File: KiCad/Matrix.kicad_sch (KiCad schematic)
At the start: 0 parts

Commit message: "finish" the keyboard schematics
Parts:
- added D1: ESC, symbol Device:D
- added D10: F9, symbol Device:D
- added D11: F10, symbol Device:D
- added D12: F11, symbol Device:D
- added D13: F12, symbol Device:D
- added D14: Del, symbol Device:D
- added D15: Ins, symbol Device:D
- added D16: `/~, symbol Device:D
- added D17: 1, symbol Device:D
- added D18: 2, symbol Device:D
- added D19: 3, symbol Device:D
- added D2: F1, symbol Device:D
- added D20: 4, symbol Device:D
- added D21: 5, symbol Device:D
- added D22: 6, symbol Device:D
- added D23: 7, symbol Device:D
- added D24: 8, symbol Device:D
- added D25: 9, symbol Device:D
- added D26: 0, symbol Device:D
- added D27: -, symbol Device:D
- added D28: +, symbol Device:D
- added D29: Backspace, symbol Device:D
- added D3: F2, symbol Device:D
- added D30: End, symbol Device:D
- added D31: Tab, symbol Device:D
- added D32: Q, symbol Device:D
- added D33: W, symbol Device:D
- added D34: E, symbol Device:D
- added D35: R, symbol Device:D
- added D36: T, symbol Device:D
- added D37: Y, symbol Device:D
- added D38: U, symbol Device:D
- added D39: I, symbol Device:D
- added D4: F3, symbol Device:D
- added D40: O, symbol Device:D
- added D41: P, symbol Device:D
- added D42: [, symbol Device:D
- added D43: ], symbol Device:D
- added D44: \, symbol Device:D
- added D45: PgUp, symbol Device:D
- added D46: CapsLock, symbol Device:D
- added D47: A, symbol Device:D
- added D48: S, symbol Device:D
- added D49: D, symbol Device:D
- added D5: F4, symbol Device:D
- added D50: F, symbol Device:D
- added D51: G, symbol Device:D
- added D52: H, symbol Device:D
- added D53: J, symbol Device:D
- added D54: K, symbol Device:D
- added D55: L, symbol Device:D
- added D56: ;, symbol Device:D
- added D57: ', symbol Device:D
- added D58: Enter, symbol Device:D
- added D59: PgDn, symbol Device:D
- added D6: F5, symbol Device:D
- added D60: LShift, symbol Device:D
- added D61: Z, symbol Device:D
- added D62: X, symbol Device:D
- added D63: C, symbol Device:D
- added D64: V, symbol Device:D
- added D65: B, symbol Device:D
- added D66: N, symbol Device:D
- added D67: M, symbol Device:D
- added D68: ,, symbol Device:D
- added D69: ., symbol Device:D
- added D7: F6, symbol Device:D
- added D70: /, symbol Device:D
- added D71: RShift, symbol Device:D
- added D72: Up, symbol Device:D
- added D73: Home, symbol Device:D
- added D74: LCtrl, symbol Device:D
- added D75: Win, symbol Device:D
- added D76, D78: Alt, symbol Device:D
- added D77: Space, symbol Device:D
- added D79: FN, symbol Device:D
- added D8: F7, symbol Device:D
- added D80: RCtrl, symbol Device:D
- added D81: Right, symbol Device:D
- added D82: Down, symbol Device:D
- added D83: Left, symbol Device:D
- added D9: F8, symbol Device:D
- added MX1, MX10, MX11, MX12, MX13, MX14, MX15, MX16, MX17, MX18, MX19, MX2, MX20, MX21, MX22, MX23, MX24, MX25, MX26, MX27, MX28, MX29, MX3, MX30, MX31, MX32, MX33, MX34, MX35, MX36, MX37, MX38, MX39, MX4, MX40, MX41, MX42, MX43, MX44, MX45, MX46, MX47, MX48, MX49, MX5, MX50, MX51, MX52, MX53, MX54, MX55, MX56, MX57, MX58, MX59, MX6, MX60, MX61, MX62, MX63, MX64, MX65, MX66, MX67, MX68, MX69, MX7, MX70, MX71, MX72, MX73, MX74, MX75, MX76, MX8, MX80, MX83, MX84, MX85, MX86, MX87, MX88, MX9: MX-NoLED, symbol MX_Alps_Hybrid:MX-NoLED
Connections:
- new net: D60.2 (A), MX59.2 (ROW)
- new net: D50.2 (A), MX50.2 (ROW)
- new net: D77.2 (A), MX80.2 (ROW)
- new net: D15.2 (A), MX15.2 (ROW)
- new net: D11.2 (A), MX11.2 (ROW)
- new net: D31.2 (A), MX31.2 (ROW)
- new net: D32.2 (A), MX32.2 (ROW)
- new net: D82.2 (A), MX87.2 (ROW)
- new net: D38.2 (A), MX38.2 (ROW)
- new net: D67.2 (A), MX67.2 (ROW)
- new net: D53.2 (A), MX53.2 (ROW)
- new net: D46.2 (A), MX46.2 (ROW)
- new net: D40.2 (A), MX40.2 (ROW)
- new net: D63.2 (A), MX63.2 (ROW)
- new net: D8.2 (A), MX8.2 (ROW)
- new net: D41.2 (A), MX41.2 (ROW)
- new net: D7.2 (A), MX7.2 (ROW)
- new net: D83.2 (A), MX88.2 (ROW)
- new net: D13.2 (A), MX13.2 (ROW)
- new net: D37.2 (A), MX37.2 (ROW)
- new net: D59.2 (A), MX60.2 (ROW)
- new net: D52.2 (A), MX52.2 (ROW)
- new net: D24.2 (A), MX24.2 (ROW)
- new net: D2.2 (A), MX2.2 (ROW)
- new net: D14.2 (A), MX14.2 (ROW)
- new net: D76.2 (A), MX76.2 (ROW)
- new net: D45.2 (A), MX45.2 (ROW)
- new net: D73.2 (A), MX74.2 (ROW)
- new net: D81.2 (A), MX86.2 (ROW)
- new net: D17.2 (A), MX17.2 (ROW)
- new net: D75.2 (A), MX75.2 (ROW)
- new net: D65.2 (A), MX65.2 (ROW)
- new net: D74.2 (A), MX71.2 (ROW)
- new net: D48.2 (A), MX48.2 (ROW)
- new net: D71.2 (A), MX72.2 (ROW)
- new net: D10.2 (A), MX10.2 (ROW)
- new net: D33.2 (A), MX33.2 (ROW)
- new net: D30.2 (A), MX30.2 (ROW)
- new net: D51.2 (A), MX51.2 (ROW)
- new net: D4.2 (A), MX4.2 (ROW)
- new net: D21.2 (A), MX21.2 (ROW)
- new net: D58.2 (A), MX58.2 (ROW)
- new net: D64.2 (A), MX64.2 (ROW)
- new net: D1.2 (A), MX1.2 (ROW)
- new net: D44.2 (A), MX44.2 (ROW)
- new net: D36.2 (A), MX36.2 (ROW)
- new net: D47.2 (A), MX47.2 (ROW)
- new net: D54.2 (A), MX54.2 (ROW)
- new net: D72.2 (A), MX73.2 (ROW)
- new net: D62.2 (A), MX62.2 (ROW)
- new net: D18.2 (A), MX18.2 (ROW)
- new net: D66.2 (A), MX66.2 (ROW)
- new net: D6.2 (A), MX6.2 (ROW)
- new net: D25.2 (A), MX25.2 (ROW)
- new net: D68.2 (A), MX68.2 (ROW)
- new net: D34.2 (A), MX34.2 (ROW)
- new net: D35.2 (A), MX35.2 (ROW)
- new net: D55.2 (A), MX55.2 (ROW)
- new net: D16.2 (A), MX16.2 (ROW)
- new net: D27.2 (A), MX27.2 (ROW)
- new net: D57.2 (A), MX57.2 (ROW)
- new net: D28.2 (A), MX28.2 (ROW)
- new net: D9.2 (A), MX9.2 (ROW)
- new net: D39.2 (A), MX39.2 (ROW)
- new net: D78.2 (A), MX83.2 (ROW)
- new net: D23.2 (A), MX23.2 (ROW)
- new net: D70.2 (A), MX70.2 (ROW)
- new net: D20.2 (A), MX20.2 (ROW)
- new net: D3.2 (A), MX3.2 (ROW)
- new net: D19.2 (A), MX19.2 (ROW)
- new net: D69.2 (A), MX69.2 (ROW)
- new net: D49.2 (A), MX49.2 (ROW)
- new net: D29.2 (A), MX29.2 (ROW)
- new net: D5.2 (A), MX5.2 (ROW)
- new net: D42.2 (A), MX42.2 (ROW)
- new net: D26.2 (A), MX26.2 (ROW)
- new net: D80.2 (A), MX85.2 (ROW)
- new net: D22.2 (A), MX22.2 (ROW)
- new net: D79.2 (A), MX84.2 (ROW)
- new net: D61.2 (A), MX61.2 (ROW)
- new net: D43.2 (A), MX43.2 (ROW)
- new net: D12.2 (A), MX12.2 (ROW)
- new net: D56.2 (A), MX56.2 (ROW)
- new net col0: MX1.1 (COL), MX16.1 (COL), MX31.1 (COL), MX46.1 (COL), MX59.1 (COL), MX71.1 (COL)
- new net col1: MX17.1 (COL), MX2.1 (COL), MX32.1 (COL), MX47.1 (COL), MX61.1 (COL), MX75.1 (COL)
- new net col10: MX11.1 (COL), MX26.1 (COL), MX41.1 (COL), MX56.1 (COL), MX70.1 (COL), MX84.1 (COL)
- new net col11: MX12.1 (COL), MX27.1 (COL), MX42.1 (COL), MX57.1 (COL), MX85.1 (COL)
- new net col12: MX13.1 (COL), MX28.1 (COL), MX43.1 (COL), MX58.1 (COL), MX72.1 (COL), MX86.1 (COL)
- new net col13: MX14.1 (COL), MX29.1 (COL), MX44.1 (COL), MX73.1 (COL), MX87.1 (COL)
- new net col14: MX15.1 (COL), MX30.1 (COL), MX45.1 (COL), MX60.1 (COL), MX74.1 (COL), MX88.1 (COL)
- new net col2: MX18.1 (COL), MX3.1 (COL), MX33.1 (COL), MX48.1 (COL), MX62.1 (COL), MX76.1 (COL)
- new net col3: MX19.1 (COL), MX34.1 (COL), MX4.1 (COL), MX49.1 (COL), MX63.1 (COL)
- new net col4: MX20.1 (COL), MX35.1 (COL), MX5.1 (COL), MX50.1 (COL), MX64.1 (COL)
- new net col5: MX21.1 (COL), MX36.1 (COL), MX51.1 (COL), MX6.1 (COL), MX65.1 (COL)
- new net col6: MX22.1 (COL), MX37.1 (COL), MX52.1 (COL), MX66.1 (COL), MX7.1 (COL), MX80.1 (COL)
- new net col7: MX23.1 (COL), MX38.1 (COL), MX53.1 (COL), MX67.1 (COL), MX8.1 (COL)
- new net col8: MX24.1 (COL), MX39.1 (COL), MX54.1 (COL), MX68.1 (COL), MX9.1 (COL)
- new net col9: MX10.1 (COL), MX25.1 (COL), MX40.1 (COL), MX55.1 (COL), MX69.1 (COL), MX83.1 (COL)
- new net row0: D1.1 (K), D10.1 (K), D11.1 (K), D12.1 (K), D13.1 (K), D14.1 (K), D15.1 (K), D2.1 (K), D3.1 (K), D4.1 (K), D5.1 (K), D6.1 (K), D7.1 (K), D8.1 (K), D9.1 (K)
- new net row1: D16.1 (K), D17.1 (K), D18.1 (K), D19.1 (K), D20.1 (K), D21.1 (K), D22.1 (K), D23.1 (K), D24.1 (K), D25.1 (K), D26.1 (K), D27.1 (K), D28.1 (K), D29.1 (K), D30.1 (K)
- new net row2: D31.1 (K), D32.1 (K), D33.1 (K), D34.1 (K), D35.1 (K), D36.1 (K), D37.1 (K), D38.1 (K), D39.1 (K), D40.1 (K), D41.1 (K), D42.1 (K), D43.1 (K), D44.1 (K), D45.1 (K)
- new net row3: D46.1 (K), D47.1 (K), D48.1 (K), D49.1 (K), D50.1 (K), D51.1 (K), D52.1 (K), D53.1 (K), D54.1 (K), D55.1 (K), D56.1 (K), D57.1 (K), D58.1 (K), D59.1 (K)
- new net row4: D60.1 (K), D61.1 (K), D62.1 (K), D63.1 (K), D64.1 (K), D65.1 (K), D66.1 (K), D67.1 (K), D68.1 (K), D69.1 (K), D70.1 (K), D71.1 (K), D72.1 (K), D73.1 (K)
- new net row5: D74.1 (K), D75.1 (K), D76.1 (K), D77.1 (K), D78.1 (K), D79.1 (K), D80.1 (K), D81.1 (K), D82.1 (K), D83.1 (K)

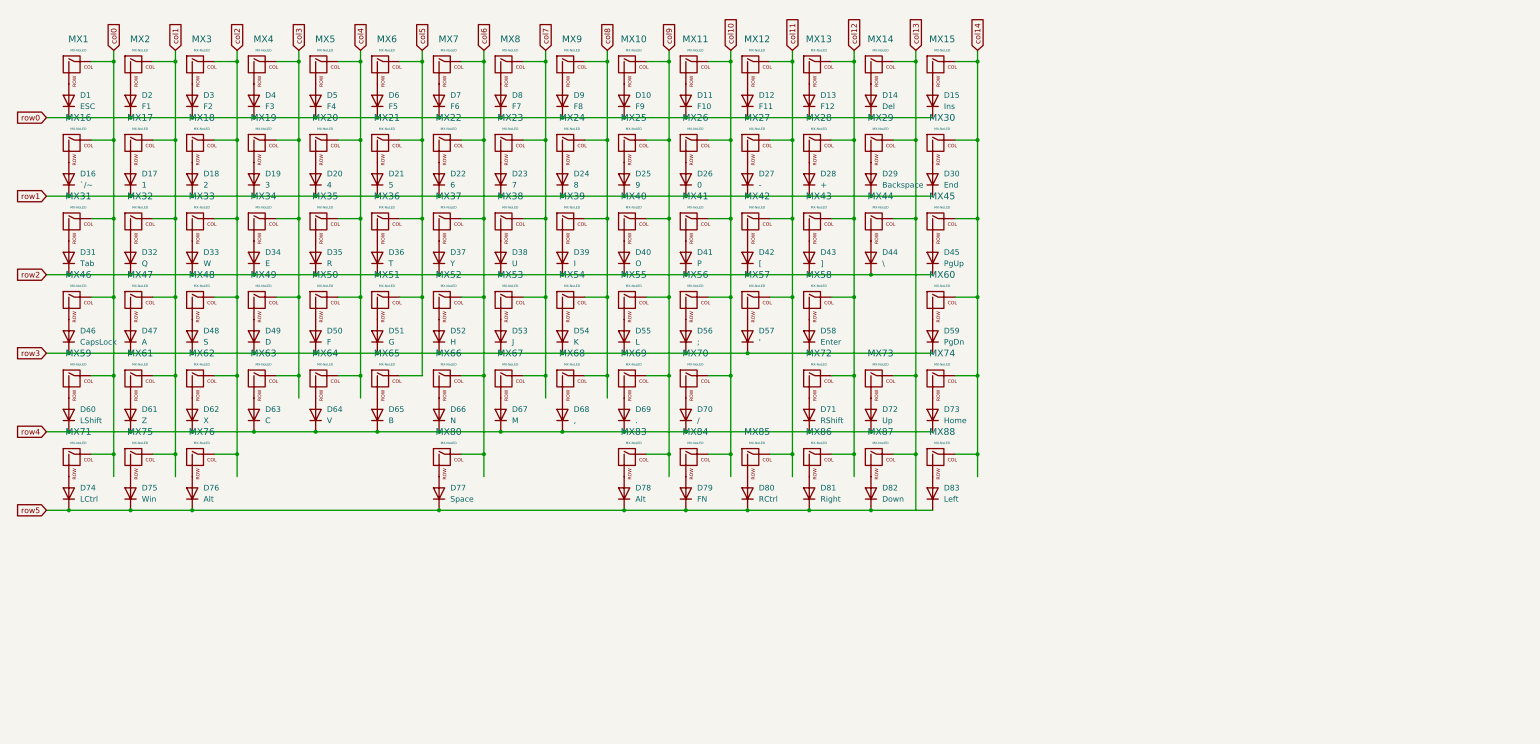
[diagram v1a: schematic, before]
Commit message: fix stuff... i forgot the other stuff i added
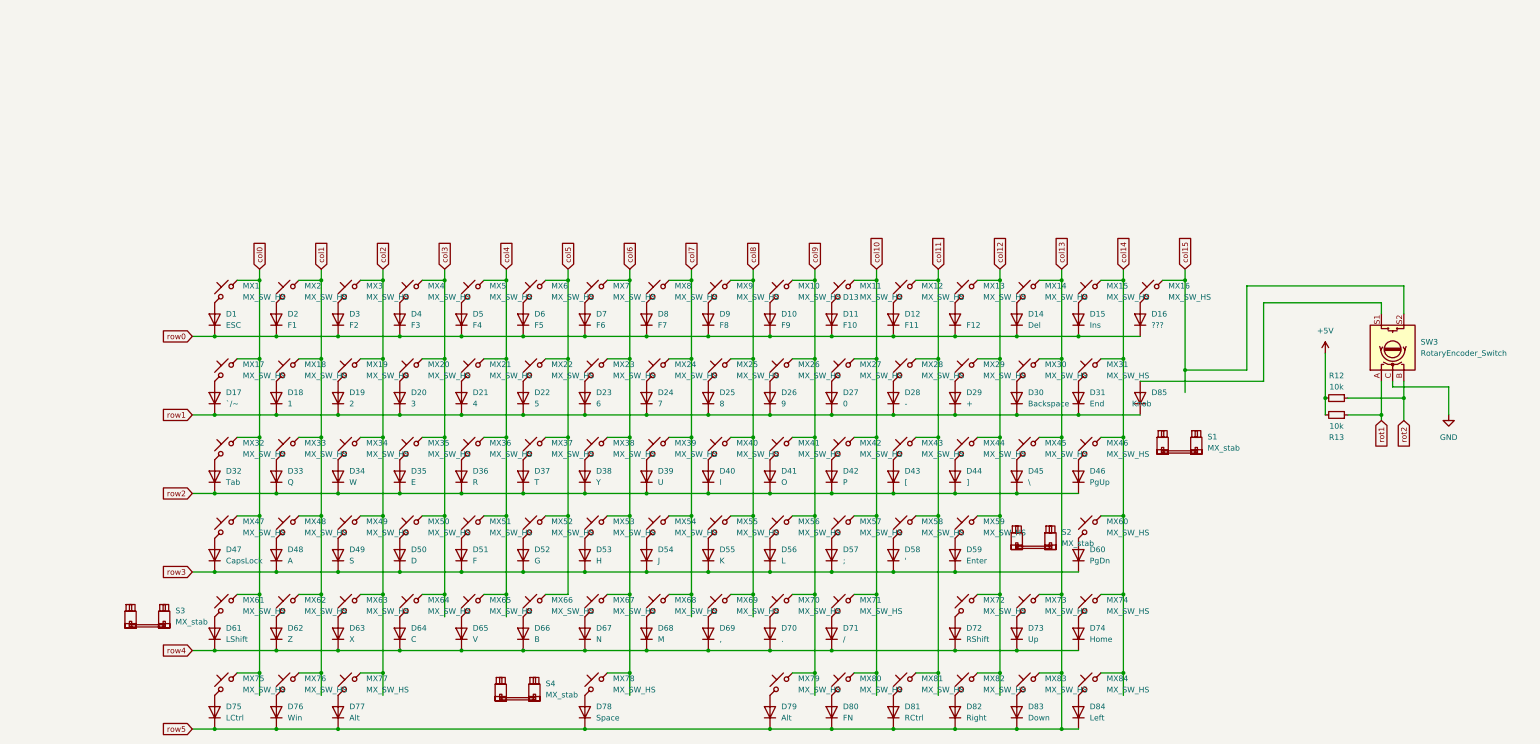
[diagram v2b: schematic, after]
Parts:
- removed MX1, MX10, MX11, MX12, MX13, MX14, MX15, MX16, MX17, MX18, MX19, MX2, MX20, MX21, MX22, MX23, MX24, MX25, MX26, MX27, MX28, MX29, MX3, MX30, MX31, MX32, MX33, MX34, MX35, MX36, MX37, MX38, MX39, MX4, MX40, MX41, MX42, MX43, MX44, MX45, MX46, MX47, MX48, MX49, MX5, MX50, MX51, MX52, MX53, MX54, MX55, MX56, MX57, MX58, MX59, MX6, MX60, MX61, MX62, MX63, MX64, MX65, MX66, MX67, MX68, MX69, MX7, MX70, MX71, MX72, MX73, MX74, MX75, MX76, MX8, MX80, MX83, MX84, MX85, MX86, MX87, MX88, MX9: MX-NoLED, symbol MX_Alps_Hybrid:MX-NoLED
- added D16: ???, Diode_SMD:D_SOD-123, symbol Device:D
- added D85: Knob, Diode_SMD:D_SOD-123, symbol Device:D
- added MX1, MX10, MX11, MX12, MX13, MX14, MX15, MX16, MX17, MX18, MX19, MX2, MX20, MX21, MX22, MX23, MX24, MX25, MX26, MX27, MX28, MX29, MX3, MX30, MX31, MX32, MX33, MX34, MX35, MX36, MX37, MX38, MX39, MX4, MX40, MX41, MX42, MX43, MX44, MX45, MX46, MX47, MX48, MX49, MX5, MX50, MX51, MX52, MX53, MX54, MX55, MX56, MX57, MX58, MX59, MX6, MX60, MX61, MX62, MX63, MX64, MX65, MX66, MX67, MX68, MX69, MX7, MX70, MX71, MX72, MX73, MX74, MX75, MX76, MX77, MX78, MX79, MX8, MX80, MX81, MX82, MX83, MX84, MX9: MX_SW_HS, PCM_marbastlib-mx:SW_MX_HS_1u, symbol PCM_marbastlib-mx:MX_SW_HS
- added R12, R13: 10k, Resistor_SMD:R_0402_1005Metric, symbol Device:R_Small
- added S1, S2, S3: MX_stab, PCM_marbastlib-mx:STAB_MX_P_2u, symbol PCM_marbastlib-mx:MX_stab
- added S4: MX_stab, PCM_marbastlib-mx:STAB_MX_P_6.25u, symbol PCM_marbastlib-mx:MX_stab
- added SW3: RotaryEncoder_Switch, Rotary_Encoder:RotaryEncoder_Alps_EC11E-Switch_Vertical_H20mm, symbol Device:RotaryEncoder_Switch
- D1, D10, D11, D12, D13, D14, D15, D2, D3, D4, D5, D6, D7, D8, D9: footprint (none) -> Diode_SMD:D_SOD-123
- D17: renamed from D16; footprint (none) -> Diode_SMD:D_SOD-123
- D18: renamed from D17; footprint (none) -> Diode_SMD:D_SOD-123
- D19: renamed from D18; footprint (none) -> Diode_SMD:D_SOD-123
- D20: renamed from D19; footprint (none) -> Diode_SMD:D_SOD-123
- D21: renamed from D20; footprint (none) -> Diode_SMD:D_SOD-123
- D22: renamed from D21; footprint (none) -> Diode_SMD:D_SOD-123
- D23: renamed from D22; footprint (none) -> Diode_SMD:D_SOD-123
- D24: renamed from D23; footprint (none) -> Diode_SMD:D_SOD-123
- D25: renamed from D24; footprint (none) -> Diode_SMD:D_SOD-123
- D26: renamed from D25; footprint (none) -> Diode_SMD:D_SOD-123
- D27: renamed from D26; footprint (none) -> Diode_SMD:D_SOD-123
- D28: renamed from D27; footprint (none) -> Diode_SMD:D_SOD-123
- D29: renamed from D28; footprint (none) -> Diode_SMD:D_SOD-123
- D30: renamed from D29; footprint (none) -> Diode_SMD:D_SOD-123
- D31: renamed from D30; footprint (none) -> Diode_SMD:D_SOD-123
- D32: renamed from D31; footprint (none) -> Diode_SMD:D_SOD-123
- D33: renamed from D32; footprint (none) -> Diode_SMD:D_SOD-123
- D34: renamed from D33; footprint (none) -> Diode_SMD:D_SOD-123
- D35: renamed from D34; footprint (none) -> Diode_SMD:D_SOD-123
- D36: renamed from D35; footprint (none) -> Diode_SMD:D_SOD-123
- D37: renamed from D36; footprint (none) -> Diode_SMD:D_SOD-123
- D38: renamed from D37; footprint (none) -> Diode_SMD:D_SOD-123
- D39: renamed from D38; footprint (none) -> Diode_SMD:D_SOD-123
- D40: renamed from D39; footprint (none) -> Diode_SMD:D_SOD-123
- D41: renamed from D40; footprint (none) -> Diode_SMD:D_SOD-123
- D42: renamed from D41; footprint (none) -> Diode_SMD:D_SOD-123
- D43: renamed from D42; footprint (none) -> Diode_SMD:D_SOD-123
- D44: renamed from D43; footprint (none) -> Diode_SMD:D_SOD-123
- D45: renamed from D44; footprint (none) -> Diode_SMD:D_SOD-123
- D46: renamed from D45; footprint (none) -> Diode_SMD:D_SOD-123
- D47: renamed from D46; footprint (none) -> Diode_SMD:D_SOD-123
- D48: renamed from D47; footprint (none) -> Diode_SMD:D_SOD-123
- D49: renamed from D48; footprint (none) -> Diode_SMD:D_SOD-123
- D50: renamed from D49; footprint (none) -> Diode_SMD:D_SOD-123
- D51: renamed from D50; footprint (none) -> Diode_SMD:D_SOD-123
- D52: renamed from D51; footprint (none) -> Diode_SMD:D_SOD-123
- D53: renamed from D52; footprint (none) -> Diode_SMD:D_SOD-123
- D54: renamed from D53; footprint (none) -> Diode_SMD:D_SOD-123
- D55: renamed from D54; footprint (none) -> Diode_SMD:D_SOD-123
- D56: renamed from D55; footprint (none) -> Diode_SMD:D_SOD-123
- D57: renamed from D56; footprint (none) -> Diode_SMD:D_SOD-123
- D58: renamed from D57; footprint (none) -> Diode_SMD:D_SOD-123
- D59: renamed from D58; footprint (none) -> Diode_SMD:D_SOD-123
- D60: renamed from D59; footprint (none) -> Diode_SMD:D_SOD-123
- D61: renamed from D60; footprint (none) -> Diode_SMD:D_SOD-123
- D62: renamed from D61; footprint (none) -> Diode_SMD:D_SOD-123
- D63: renamed from D62; footprint (none) -> Diode_SMD:D_SOD-123
- D64: renamed from D63; footprint (none) -> Diode_SMD:D_SOD-123
- D65: renamed from D64; footprint (none) -> Diode_SMD:D_SOD-123
- D66: renamed from D65; footprint (none) -> Diode_SMD:D_SOD-123
- D67: renamed from D66; footprint (none) -> Diode_SMD:D_SOD-123
- D68: renamed from D67; footprint (none) -> Diode_SMD:D_SOD-123
- D69: renamed from D68; footprint (none) -> Diode_SMD:D_SOD-123
- D70: renamed from D69; footprint (none) -> Diode_SMD:D_SOD-123
- D71: renamed from D70; footprint (none) -> Diode_SMD:D_SOD-123
- D72: renamed from D71; footprint (none) -> Diode_SMD:D_SOD-123
- D73: renamed from D72; footprint (none) -> Diode_SMD:D_SOD-123
- D74: renamed from D73; footprint (none) -> Diode_SMD:D_SOD-123
- D75: renamed from D74; footprint (none) -> Diode_SMD:D_SOD-123
- D76: renamed from D75; footprint (none) -> Diode_SMD:D_SOD-123
- D77: renamed from D76; footprint (none) -> Diode_SMD:D_SOD-123
- D78: renamed from D77; footprint (none) -> Diode_SMD:D_SOD-123
- D79: renamed from D78; footprint (none) -> Diode_SMD:D_SOD-123
- D80: renamed from D79; footprint (none) -> Diode_SMD:D_SOD-123
- D81: renamed from D80; footprint (none) -> Diode_SMD:D_SOD-123
- D82: renamed from D81; footprint (none) -> Diode_SMD:D_SOD-123
- D83: renamed from D82; footprint (none) -> Diode_SMD:D_SOD-123
- D84: renamed from D83; footprint (none) -> Diode_SMD:D_SOD-123
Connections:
- net row5 is gone; now on net col13: D75.1 (K), D76.1 (K), D77.1 (K), D78.1 (K), D79.1 (K), D80.1 (K), D81.1 (K), D82.1 (K), D83.1 (K), D84.1 (K)
- net col0: now also MX1.2, MX17.2, MX32.2, MX47.2, MX61.2, MX75.2
- net col1: now also MX18.2, MX2.2, MX33.2, MX48.2, MX62.2, MX76.2
- net col10: now also MX11.2, MX27.2, MX42.2, MX57.2, MX71.2, MX80.2
- net col11: now also MX12.2, MX28.2, MX43.2, MX58.2, MX81.2
- net col12: now also MX13.2, MX29.2, MX44.2, MX59.2, MX72.2, MX82.2
- net col13: now also MX14.2, MX30.2, MX45.2, MX73.2, MX83.2
- net col14: now also MX15.2, MX31.2, MX46.2, MX60.2, MX74.2, MX84.2
- net col2: now also MX19.2, MX3.2, MX34.2, MX49.2, MX63.2, MX77.2
- net col3: now also MX20.2, MX35.2, MX4.2, MX50.2, MX64.2
- net col4: now also MX21.2, MX36.2, MX5.2, MX51.2, MX65.2
- net col5: now also MX22.2, MX37.2, MX52.2, MX6.2, MX66.2
- net col6: now also MX23.2, MX38.2, MX53.2, MX67.2, MX7.2, MX78.2
- net col7: now also MX24.2, MX39.2, MX54.2, MX68.2, MX8.2
- net col8: now also MX25.2, MX40.2, MX55.2, MX69.2, MX9.2
- net col9: now also MX10.2, MX26.2, MX41.2, MX56.2, MX70.2, MX79.2
- net row0: now also D16.1 (K)
- net row1: now also D85.1 (K)
- net at D61.2 (A): now also MX61.1
- net at D51.2 (A): now also MX51.1
- net at D78.2 (A): now also MX78.1
- net at D15.2 (A): now also MX15.1
- net at D11.2 (A): now also MX11.1
- net at D32.2 (A): now also MX32.1
- net at D33.2 (A): now also MX33.1
- net at D83.2 (A): now also MX83.1
- net at D39.2 (A): now also MX39.1
- net at D68.2 (A): now also MX68.1
- net at D54.2 (A): now also MX54.1
- net at D47.2 (A): now also MX47.1
- net at D41.2 (A): now also MX41.1
- net at D64.2 (A): now also MX64.1
- net at D8.2 (A): now also MX8.1
- net at D42.2 (A): now also MX42.1
- net at D7.2 (A): now also MX7.1
- net at D84.2 (A): now also MX84.1
- net at D13.2 (A): now also MX13.1
- net at D38.2 (A): now also MX38.1
- net at D60.2 (A): now also MX60.1
- net at D53.2 (A): now also MX53.1
- net at D25.2 (A): now also MX25.1
- net at D2.2 (A): now also MX2.1
- net at D14.2 (A): now also MX14.1
- net at D77.2 (A): now also MX77.1
- net at D46.2 (A): now also MX46.1
- net at D74.2 (A): now also MX74.1
- net at D82.2 (A): now also MX82.1
- net at D18.2 (A): now also MX18.1
- net at D76.2 (A): now also MX76.1
- net at D66.2 (A): now also MX66.1
- net at D75.2 (A): now also MX75.1
- net at D49.2 (A): now also MX49.1
- net at D72.2 (A): now also MX72.1
- net at D10.2 (A): now also MX10.1
- net at D34.2 (A): now also MX34.1
- net at D31.2 (A): now also MX31.1
- net at D52.2 (A): now also MX52.1
- net at D4.2 (A): now also MX4.1
- net at D22.2 (A): now also MX22.1
- net at D59.2 (A): now also MX59.1
- net at D65.2 (A): now also MX65.1
- net at D1.2 (A): now also MX1.1
- net at D45.2 (A): now also MX45.1
- net at D37.2 (A): now also MX37.1
- net at D48.2 (A): now also MX48.1
- net at D55.2 (A): now also MX55.1
- net at D73.2 (A): now also MX73.1
- net at D63.2 (A): now also MX63.1
- net at D19.2 (A): now also MX19.1
- net at D67.2 (A): now also MX67.1
- net at D6.2 (A): now also MX6.1
- net at D26.2 (A): now also MX26.1
- net at D69.2 (A): now also MX69.1
- net at D35.2 (A): now also MX35.1
- net at D36.2 (A): now also MX36.1
- net at D56.2 (A): now also MX56.1
- net at D17.2 (A): now also MX17.1
- net at D28.2 (A): now also MX28.1
- net at D58.2 (A): now also MX58.1
- net at D29.2 (A): now also MX29.1
- net at D9.2 (A): now also MX9.1
- net at D40.2 (A): now also MX40.1
- net at D79.2 (A): now also MX79.1
- net at D24.2 (A): now also MX24.1
- net at D71.2 (A): now also MX71.1
- net at D21.2 (A): now also MX21.1
- net at D3.2 (A): now also MX3.1
- net at D20.2 (A): now also MX20.1
- net at D70.2 (A): now also MX70.1
- net at D50.2 (A): now also MX50.1
- net at D30.2 (A): now also MX30.1
- net at D5.2 (A): now also MX5.1
- net at D43.2 (A): now also MX43.1
- net at D27.2 (A): now also MX27.1
- net at D81.2 (A): now also MX81.1
- net at D23.2 (A): now also MX23.1
- net at D80.2 (A): now also MX80.1
- net at D62.2 (A): now also MX62.1
- net at D44.2 (A): now also MX44.1
- net at D12.2 (A): now also MX12.1
- net at D57.2 (A): now also MX57.1
- new net: D16.2 (A), MX16.1
- new net: D85.2 (A), SW3.S1
- new net +5V: R12.2, R13.2
- new net GND: SW3.C
- new net col15: MX16.2, SW3.S2
- new net rot1: R13.1, SW3.A
- new net rot2: R12.1, SW3.B
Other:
- moved on the sheet: D1, D10, D11, D12, D13, D14, D15, D17, D18, D19, D2, D20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
